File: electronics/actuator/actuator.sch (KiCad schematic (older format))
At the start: 34 parts, among them J1 MOTOR_OUT, J2 PWR_IN, J3 Pinouts, J4 Pinouts, Q1 NTMFS4935NT1G, Q2 NTMFS4935NT1G, Q3 NTMFS4935NT1G, Q4 NTMFS4935NT1G, Q5 NTMFS4935NT1G, Q6 NTMFS4935NT1G, U1 drv8323rs

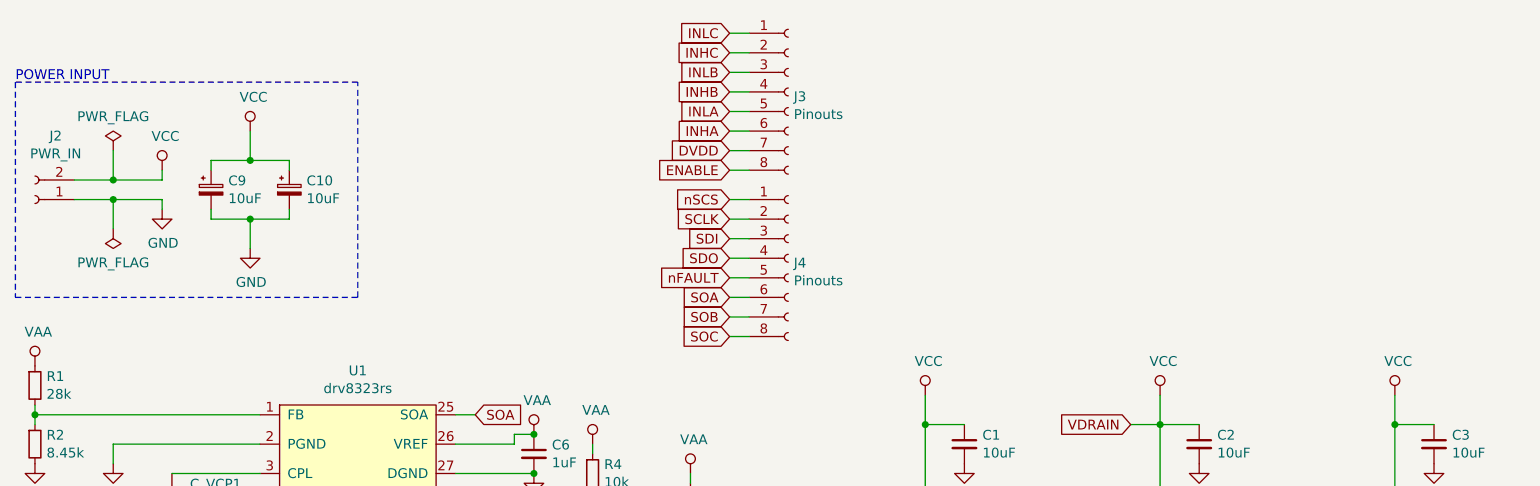
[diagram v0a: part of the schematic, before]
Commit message: Finished pcb.
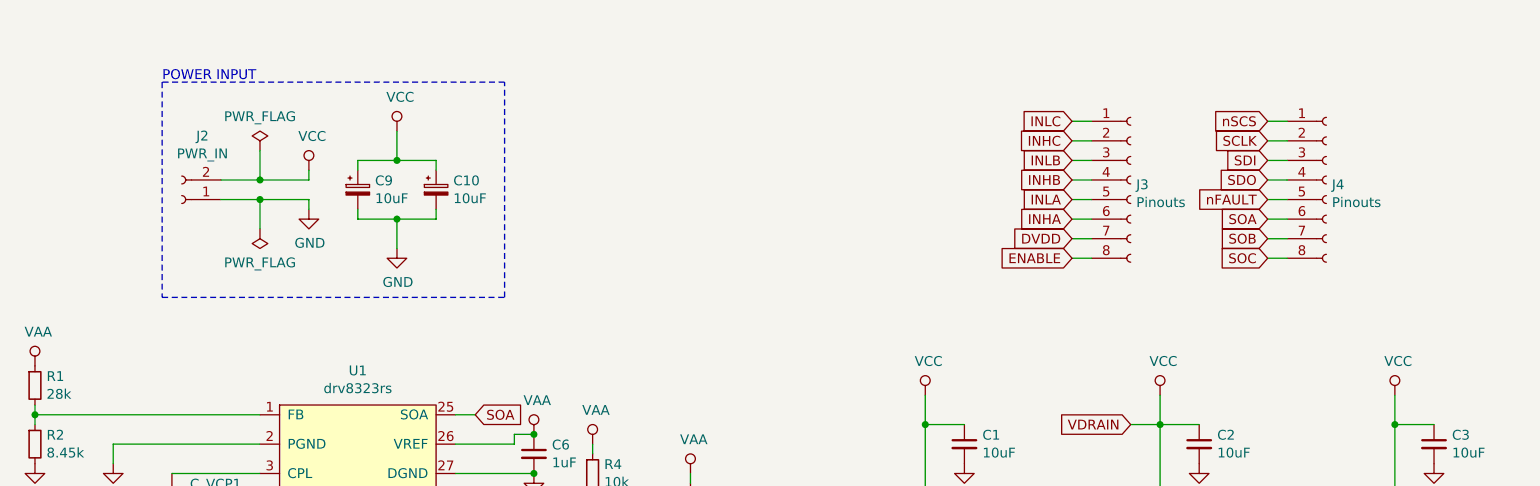
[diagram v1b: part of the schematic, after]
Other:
- moved on the sheet: C10, C9, J2, J3, J4

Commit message: Finished board.
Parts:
- U1: footprint Package_DFN_QFN:Texas_S-PVQFN-N48_EP5.15x5.15mm_ThermalVias -> actuator:Texas_S-PVQFN-N48_EP5.15x5.15mm_ThermalVias
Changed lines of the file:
@@
 F 0 "U1" H 2700 5225 50  0000 C CNN
 F 1 "drv8323rs" H 2700 5134 50  0000 C CNN
-F 2 "Package_DFN_QFN:Texas_S-PVQFN-N48_EP5.15x5.15mm_ThermalVias" H 2700 3850 50  0001 C CNN
+F 2 "actuator:Texas_S-PVQFN-N48_EP5.15x5.15mm_ThermalVias" H 2700 3850 50  0001 C CNN
 F 3 "" H 2700 3850 50  0001 C CNN
 	1    2700 3850
@@
 $EndComp
 $Comp
-L power:VCC #PWR?
+L power:VCC #PWR0107
 U 1 1 5D6883AB
 P 5600 2600
-F 0 "#PWR?" H 5600 2450 50  0001 C CNN
+F 0 "#PWR0107" H 5600 2450 50  0001 C CNN
 F 1 "VCC" H 5617 2773 50  0000 C CNN
 F 2 "" H 5600 2600 50  0001 C CNN
@@
 $EndComp
 $Comp
-L power:VCC #PWR?
+L power:VCC #PWR0108
 U 1 1 5D688401
 P 6800 2600
-F 0 "#PWR?" H 6800 2450 50  0001 C CNN
+F 0 "#PWR0108" H 6800 2450 50  0001 C CNN
 F 1 "VCC" H 6817 2773 50  0000 C CNN
 F 2 "" H 6800 2600 50  0001 C CNN
@@
 $EndComp
 $Comp
-L power:VCC #PWR?
+L power:VCC #PWR0109
 U 1 1 5D68851C
 P 8000 2600
-F 0 "#PWR?" H 8000 2450 50  0001 C CNN
+F 0 "#PWR0109" H 8000 2450 50  0001 C CNN
 F 1 "VCC" H 8017 2773 50  0000 C CNN
 F 2 "" H 8000 2600 50  0001 C CNN

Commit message: Updated board.
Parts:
- C1, C2, C3, C7, C8: footprint Capacitor_SMD:C_0603_1608Metric -> Capacitor_SMD:C_1206_3216Metric
- C10, C9: footprint Capacitor_SMD:C_0603_1608Metric -> Capacitor_SMD:CP_Elec_6.3x5.4
- L1: footprint Inductor_SMD:L_1210_3225Metric -> Inductor_THT:L_Radial_D7.8mm_P5.00mm_Fastron_07HCP
- R2: footprint Resistor_SMD:R_0603_1608Metric_Pad1.05x0.95mm_HandSolder -> Resistor_SMD:R_0402_1005Metric
- R6, R7, R8: footprint Resistor_SMD:R_1210_3225Metric -> Resistor_SMD:R_2512_6332Metric
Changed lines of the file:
@@
 F 0 "R6" H 5670 4646 50  0000 L CNN
 F 1 "1m" H 5670 4555 50  0000 L CNN
-F 2 "Resistor_SMD:R_1210_3225Metric" V 5530 4600 50  0001 C CNN
+F 2 "Resistor_SMD:R_2512_6332Metric" V 5530 4600 50  0001 C CNN
 F 3 "~" H 5600 4600 50  0001 C CNN
 	1    5600 4600
@@
 F 0 "R7" H 6870 4646 50  0000 L CNN
 F 1 "1m" H 6870 4555 50  0000 L CNN
-F 2 "Resistor_SMD:R_1210_3225Metric" V 6730 4600 50  0001 C CNN
+F 2 "Resistor_SMD:R_2512_6332Metric" V 6730 4600 50  0001 C CNN
 F 3 "~" H 6800 4600 50  0001 C CNN
 	1    6800 4600
@@
 F 0 "R8" H 8070 4646 50  0000 L CNN
 F 1 "1m" H 8070 4555 50  0000 L CNN
-F 2 "Resistor_SMD:R_1210_3225Metric" V 7930 4600 50  0001 C CNN
+F 2 "Resistor_SMD:R_2512_6332Metric" V 7930 4600 50  0001 C CNN
 F 3 "~" H 8000 4600 50  0001 C CNN
 	1    8000 4600
@@
 F 0 "R2" H 1109 2896 50  0000 L CNN
 F 1 "8.45k" H 1109 2805 50  0000 L CNN
-F 2 "Resistor_SMD:R_0603_1608Metric_Pad1.05x0.95mm_HandSolder" H 1050 2850 50  0001 C CNN
+F 2 "Resistor_SMD:R_0402_1005Metric" H 1050 2850 50  0001 C CNN
 F 3 "~" H 1050 2850 50  0001 C CNN
 	1    1050 2850
@@
 F 0 "L1" V 4100 5700 50  0000 C CNN
 F 1 "27uH" V 4200 5700 50  0000 C CNN
-F 2 "Inductor_SMD:L_1210_3225Metric" H 4250 5700 50  0001 C CNN
+F 2 "Inductor_THT:L_Radial_D7.8mm_P5.00mm_Fastron_07HCP" H 4250 5700 50  0001 C CNN
 F 3 "~" H 4250 5700 50  0001 C CNN
 	1    4250 5700
@@
 F 0 "C8" H 4642 5846 50  0000 L CNN
 F 1 "10uF" H 4642 5755 50  0000 L CNN
-F 2 "Capacitor_SMD:C_0603_1608Metric" H 4550 5800 50  0001 C CNN
+F 2 "Capacitor_SMD:C_1206_3216Metric" H 4550 5800 50  0001 C CNN
 F 3 "~" H 4550 5800 50  0001 C CNN
 	1    4550 5800
@@
 F 0 "C7" H 3792 6296 50  0000 L CNN
 F 1 "10uF" H 3792 6205 50  0000 L CNN
-F 2 "Capacitor_SMD:C_0603_1608Metric" H 3700 6250 50  0001 C CNN
+F 2 "Capacitor_SMD:C_1206_3216Metric" H 3700 6250 50  0001 C CNN
 F 3 "~" H 3700 6250 50  0001 C CNN
 	1    3700 6250
@@
 F 0 "C10" H 3188 1596 50  0000 L CNN
 F 1 "10uF" H 3188 1505 50  0000 L CNN
-F 2 "Capacitor_SMD:C_0603_1608Metric" H 3100 1550 50  0001 C CNN
+F 2 "Capacitor_SMD:CP_Elec_6.3x5.4" H 3100 1550 50  0001 C CNN
 F 3 "~" H 3100 1550 50  0001 C CNN
 	1    3100 1550
@@
 F 0 "C9" H 2788 1596 50  0000 L CNN
 F 1 "10uF" H 2788 1505 50  0000 L CNN
-F 2 "Capacitor_SMD:C_0603_1608Metric" H 2700 1550 50  0001 C CNN
+F 2 "Capacitor_SMD:CP_Elec_6.3x5.4" H 2700 1550 50  0001 C CNN
 F 3 "~" H 2700 1550 50  0001 C CNN
 	1    2700 1550
@@
 F 0 "C1" H 5892 2896 50  0000 L CNN
 F 1 "10uF" H 5892 2805 50  0000 L CNN
-F 2 "Capacitor_SMD:C_0603_1608Metric" H 5800 2850 50  0001 C CNN
+F 2 "Capacitor_SMD:C_1206_3216Metric" H 5800 2850 50  0001 C CNN
 F 3 "~" H 5800 2850 50  0001 C CNN
 	1    5800 2850
@@
 F 0 "C2" H 7092 2896 50  0000 L CNN
 F 1 "10uF" H 7092 2805 50  0000 L CNN
-F 2 "Capacitor_SMD:C_0603_1608Metric" H 7000 2850 50  0001 C CNN
+F 2 "Capacitor_SMD:C_1206_3216Metric" H 7000 2850 50  0001 C CNN
 F 3 "~" H 7000 2850 50  0001 C CNN
 	1    7000 2850
@@
 F 0 "C3" H 8292 2896 50  0000 L CNN
 F 1 "10uF" H 8292 2805 50  0000 L CNN
-F 2 "Capacitor_SMD:C_0603_1608Metric" H 8200 2850 50  0001 C CNN
+F 2 "Capacitor_SMD:C_1206_3216Metric" H 8200 2850 50  0001 C CNN
 F 3 "~" H 8200 2850 50  0001 C CNN
 	1    8200 2850
